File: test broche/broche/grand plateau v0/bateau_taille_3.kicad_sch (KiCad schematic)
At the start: 2 parts

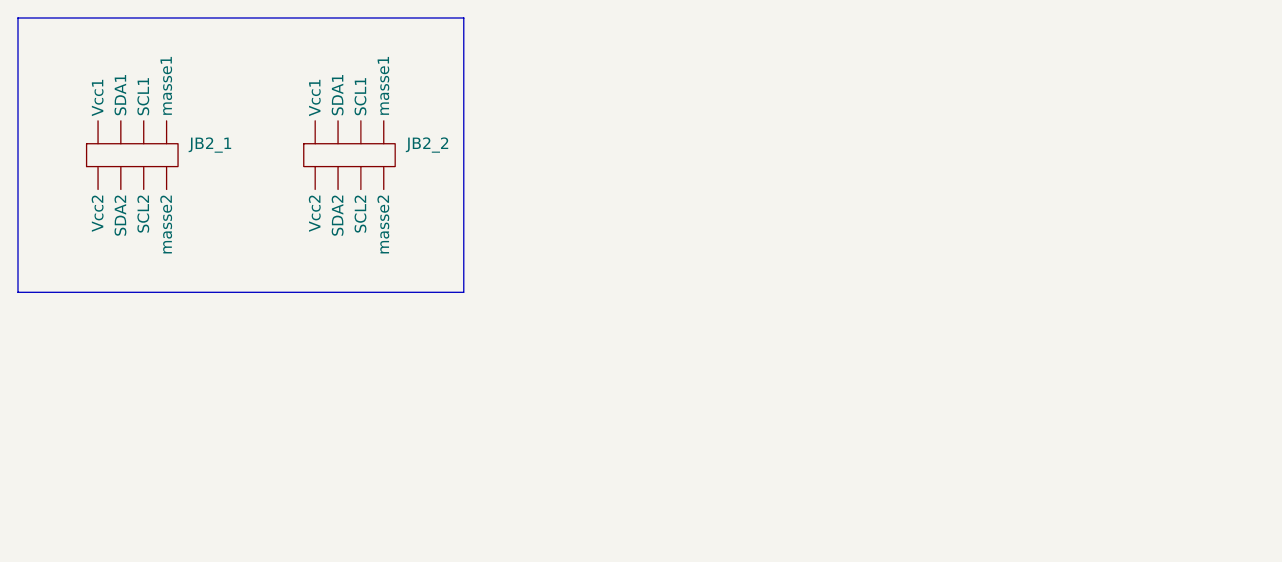
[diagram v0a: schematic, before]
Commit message: bateaux
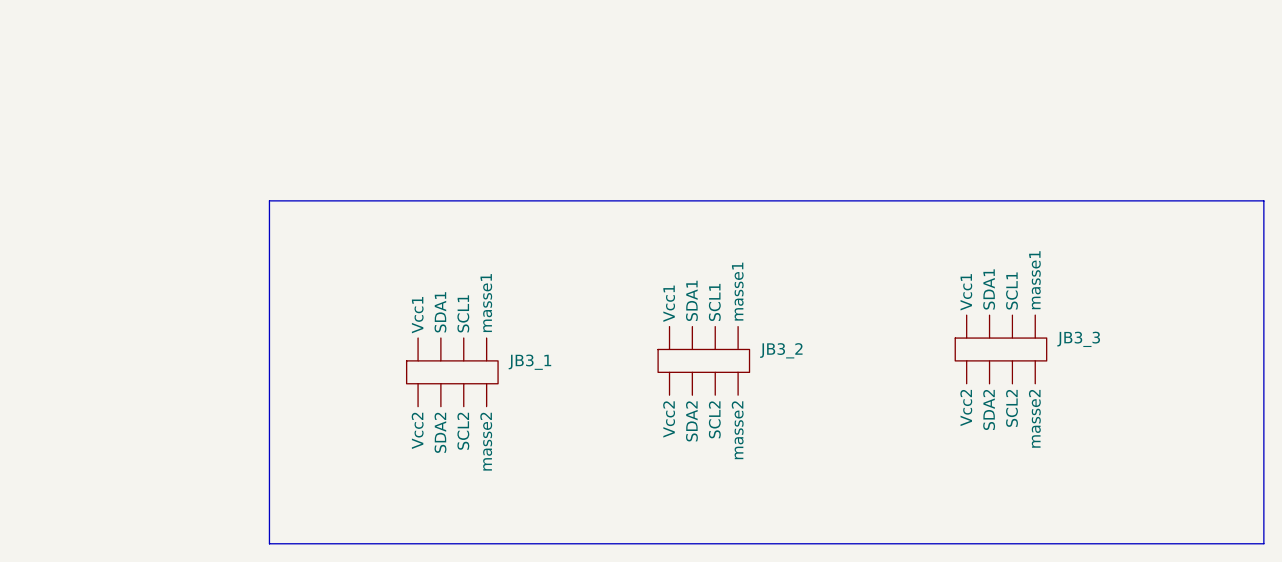
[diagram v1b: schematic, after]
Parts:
- removed JB2_1, JB2_2: ~, Mes_empreintes:Untitled, symbol Mes_symboles:Conn_rond_8_1
- added JB3_1, JB3_2, JB3_3: ~, symbol Mes_symboles:Conn_rond_8_1
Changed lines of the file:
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@@
 	(paper "A4")
 	(rectangle
-		(start 48.26 64.77)
-		(end 97.79 95.25)
+		(start 76.2 85.09)
+		(end 186.69 123.19)
 		(stroke
 			(width 0)
@@
 	)
 	(symbol
-		(lib_name "Conn_rond_8_1_2")
 		(lib_id "Mes_symboles:Conn_rond_8_1")
-		(at 60.96 81.28 0)
+		(at 96.52 105.41 0)
 		(unit 1)
 		(exclude_from_sim no)
@@
 		(dnp no)
 		(fields_autoplaced yes)
-		(property "Reference" "JB2_1"
-			(at 67.31 78.7399 0)
+		(property "Reference" "JB3_1"
+			(at 102.87 102.8699 0)
 			(effects
 				(font
@@
 		)
 		(property "Value" "~"
-			(at 67.31 81.2799 0)
-			(effects
-				(font
-					(size 1.27 1.27)
-				)
-				(justify left)
-			)
-		)
-		(property "Footprint" "Mes_empreintes:Untitled"
-			(at 60.96 81.28 0)
+			(at 102.87 105.4099 0)
+			(effects
+				(font
+					(size 1.27 1.27)
+				)
+				(justify left)
+			)
+		)
+		(property "Footprint" ""
+			(at 96.52 105.41 0)
 			(effects
 				(font
@@
 		)
 		(property "Datasheet" ""
-			(at 60.96 81.28 0)
+			(at 96.52 105.41 0)
 			(effects
 				(font
@@
 		)
 		(property "Description" ""
-			(at 60.96 81.28 0)
+			(at 96.52 105.41 0)
 			(effects
 				(font
@@
 		)
 		(instances
-			(project "grand plateau v0"
-				(path "/7a85495e-2bfc-48e4-8ed7-0a3f11b4bc2f/42a30afe-4a98-4827-8d2f-353789b9fe3f"
-					(reference "JB2_1")
+			(project ""
+				(path "/7a85495e-2bfc-48e4-8ed7-0a3f11b4bc2f/26c10166-d065-456d-a9ec-e373476587a8"
+					(reference "JB3_1")
 					(unit 1)
 				)
@@
 	)
 	(symbol
-		(lib_name "Conn_rond_8_1_1")
+		(lib_name "Conn_rond_8_1_2")
 		(lib_id "Mes_symboles:Conn_rond_8_1")
-		(at 85.09 81.28 0)
+		(at 157.48 102.87 0)
 		(unit 1)
 		(exclude_from_sim no)
@@
 		(dnp no)
 		(fields_autoplaced yes)
-		(property "Reference" "JB2_2"
-			(at 91.44 78.7399 0)
+		(property "Reference" "JB3_3"
+			(at 163.83 100.3299 0)
 			(effects
 				(font
@@
 		)
 		(property "Value" "~"
-			(at 91.44 81.2799 0)
-			(effects
-				(font
-					(size 1.27 1.27)
-				)
-				(justify left)
-			)
-		)
-		(property "Footprint" "Mes_empreintes:Untitled"
-			(at 85.09 81.28 0)
+			(at 163.83 102.8699 0)
+			(effects
+				(font
+					(size 1.27 1.27)
+				)
+				(justify left)
+			)
+		)
+		(property "Footprint" ""
+			(at 157.48 102.87 0)
 			(effects
 				(font
@@
 		)
 		(property "Datasheet" ""
-			(at 85.09 81.28 0)
+			(at 157.48 102.87 0)
 			(effects
 				(font
@@
 		)
 		(property "Description" ""
-			(at 85.09 81.28 0)
+			(at 157.48 102.87 0)
 			(effects
 				(font
@@
 		)
 		(instances
-			(project "grand plateau v0"
-				(path "/7a85495e-2bfc-48e4-8ed7-0a3f11b4bc2f/42a30afe-4a98-4827-8d2f-353789b9fe3f"
-					(reference "JB2_2")
+			(project ""
+				(path "/7a85495e-2bfc-48e4-8ed7-0a3f11b4bc2f/26c10166-d065-456d-a9ec-e373476587a8"
+					(reference "JB3_3")
 					(unit 1)
 				)
+			)
+		)
+	)
+	(symbol
+		(lib_name "Conn_rond_8_1_1")
+		(lib_id "Mes_symboles:Conn_rond_8_1")
+		(at 124.46 104.14 0)
+		(unit 1)
+		(exclude_from_sim no)
+		(in_bom yes)
+		(on_board yes)
+		(dnp no)
+		(fields_autoplaced yes)
+		(property "Reference" "JB3_2"
+			(at 130.81 101.5999 0)
+			(effects
+				(font
+					(size 1.27 1.27)
+				)
+				(justify left)
+			)
+		)
+		(property "Value" "~"
+			(at 130.81 104.1399 0)
+			(effects
+				(font
+					(size 1.27 1.27)
+				)
+				(justify left)
+			)
+		)
+		(property "Footprint" ""
+			(at 124.46 104.14 0)
+			(effects
+				(font
+					(size 1.27 1.27)
+				)
+				(hide yes)
+			)
+		)
+		(property "Datasheet" ""
+			(at 124.46 104.14 0)
+			(effects
+				(font
+					(size 1.27 1.27)
+				)
+				(hide yes)
+			)
+		)
+		(property "Description" ""
+			(at 124.46 104.14 0)
+			(effects
+				(font
+					(size 1.27 1.27)
+				)
+				(hide yes)
+			)
+		)
+		(pin ""
+		)
+		(pin ""
+		)
+		(pin ""
+		)
+		(pin ""
+		)
+		(pin ""
+		)
+		(pin ""
+		)
+		(pin ""
+		)
+		(pin ""
+		)
+		(instances
+			(project ""
+				(path "/7a85495e-2bfc-48e4-8ed7-0a3f11b4bc2f/26c10166-d065-456d-a9ec-e373476587a8"
+					(reference "JB3_2")
+					(unit 1)
+				)
